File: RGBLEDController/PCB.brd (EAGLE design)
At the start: 97.5 x 48.2 mm, 21 parts, among them T1 TIP122, T2 TIP122, T3 TIP122, T4 TIP122

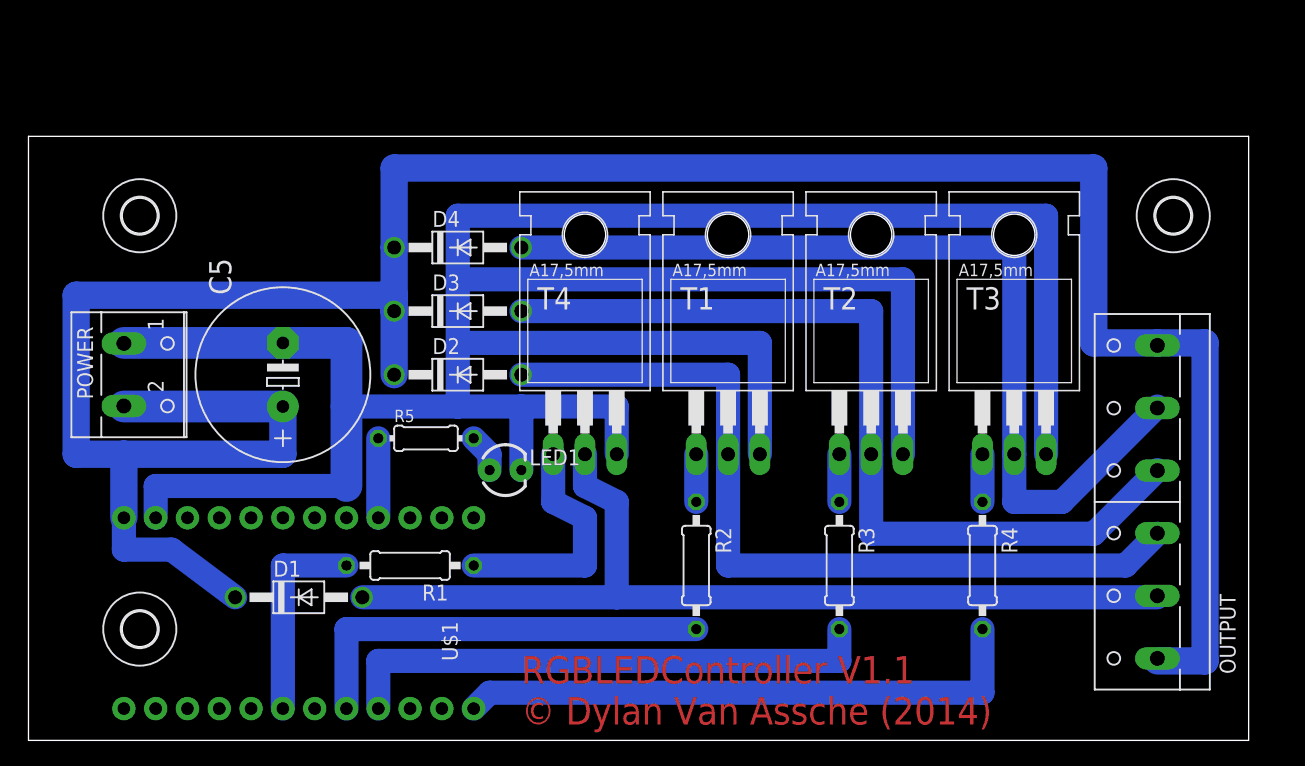
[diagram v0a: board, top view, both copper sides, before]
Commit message: V1.2
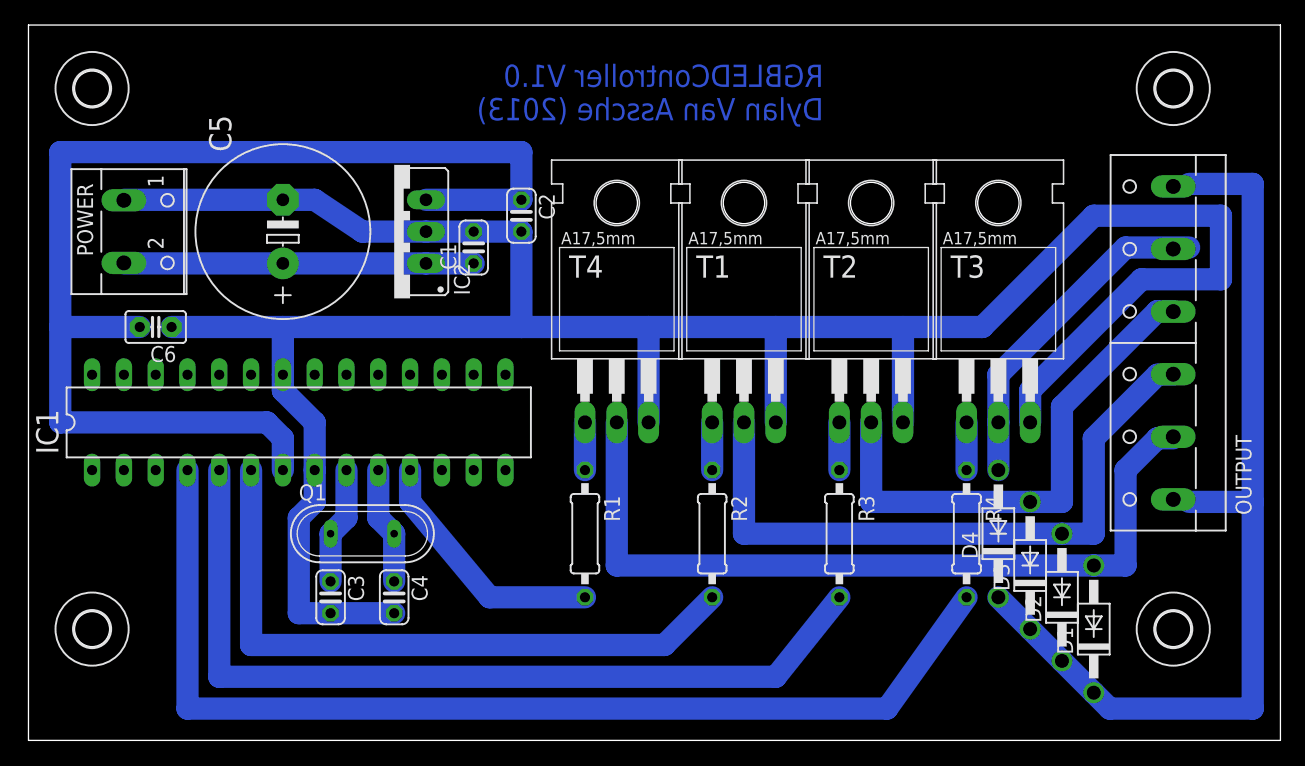
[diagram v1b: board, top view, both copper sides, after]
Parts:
- removed LED1: DAY/NIGHT, SparkFun-LED:LED3MM
- removed R5: 220, resistor:0204/7
- removed U$1: ARDUINO_PRO_MICRO, SparkFun-Boards:ARDUINO_PRO_MICRO
- added C1, C2, C3, C4: (no value), rcl:C025-024X044
- added C6: (no value), capacitor-wima:C2.5-2
- added H1: MOUNT-HOLE2.8, holes:2,8
- added IC1: ATMEGA168-PU, Arduino-AVR:DIL28-3
- added IC2: (no value), v-reg:78XXS
- added Q1: (no value), special:QS
- moved D1 63.6 mm to (85.1, 8.89), turned to 90 degrees
- moved D2 51.4 mm to (82.5, 11.4), turned to 90 degrees
- moved D3 50.0 mm to (80.0, 14.0), turned to 90 degrees
- moved D4 48.9 mm to (77.5, 16.5), turned to 90 degrees
- moved R1 14.2 mm to (44.5, 16.5), turned to 270 degrees
- moved OUTPUT 12.8 mm to (90.2, 31.8)
- moved C5 11.4 mm to (20.3, 40.6)
- moved POWER 11.4 mm to (8.89, 40.6)
- moved H3 10.9 mm to (5.08, 52.1)
- moved H4 10.2 mm to (91.4, 52.1)
- moved H2 3.81 mm to (5.08, 8.89)
- moved T4 3.59 mm to (47.0, 31.8)
- moved R2 2.84 mm to (54.6, 16.5)
- moved R4 2.84 mm to (74.9, 16.5)
- moved T1 2.84 mm to (57.1, 31.8)
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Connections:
- removed net N$3: C5.+, D1.C, D2.C, D3.C, D4.C, OUTPUT.1, OUTPUT.6, POWER.2, U$1.24
- new net N$14: IC1.5, R3.2
- new net VCC: C2.1, C6.2, IC1.20, IC1.7, IC2.OUT
- net GND: now also C1.2, C2.2, C3.2, C4.2, C6.1, IC1.22, IC1.8, IC2.GND; no longer LED1.K, U$1.23
- net N$1: now also C1.1, C5.+, D1.C, D2.C, D3.C, D4.C, IC2.IN, OUTPUT.1, OUTPUT.6, POWER.2; no longer LED1.A, R5.2
- net N$13: now also IC1.4, R4.2; no longer R5.1, U$1.16
- net N$15: now also IC1.6; no longer U$1.8
- net N$16: now also IC1.11; no longer U$1.6
- net N$5: now also C4.1, IC1.10, Q1.2; no longer R4.2, U$1.12
- net N$6: now also C3.1, IC1.9, Q1.1; no longer R3.2, U$1.9
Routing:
- net N$3: track 214.6 -> 0.00 mm
- net N$1: track 3.07 -> 104.0 mm
- net VCC: track 0.00 -> 97.0 mm
- net N$13: track 6.35 -> 85.9 mm
- net N$14: track 0.00 -> 69.1 mm
- net N$4: track 74.3 -> 27.1 mm
- net N$5: track 46.2 -> 9.42 mm
- net N$6: track 43.2 -> 9.42 mm
- net GND: track 241.3 -> 209.1 mm
- net N$7: track 70.7 -> 41.3 mm
- net N$15: track 34.3 -> 52.4 mm
- net N$12: track 19.3 -> 3.81 mm
- net N$8: track 67.1 -> 52.9 mm
- net N$9: track 76.5 -> 64.6 mm
- net N$16: track 16.5 -> 20.1 mm
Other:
- board size 97.5 x 48.2 mm -> 100 x 57.1 mm
- board text added: "RGBLEDController V1.0 Dylan Van Assche (2013)"
- board text removed: "RGBLEDController V1.1 © Dylan Van Assche (2014)"
